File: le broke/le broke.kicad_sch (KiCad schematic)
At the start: 38 parts, among them SW1 SW_Push, U1 ProMicro

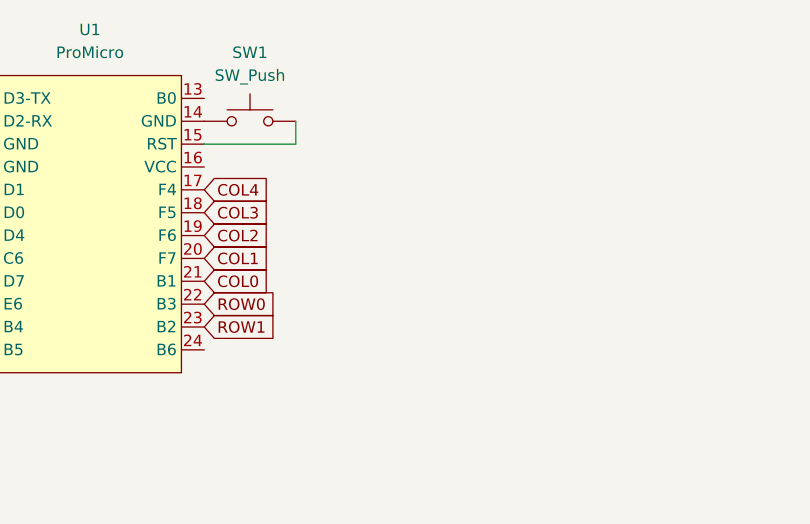
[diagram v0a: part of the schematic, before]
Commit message: new pcb etc
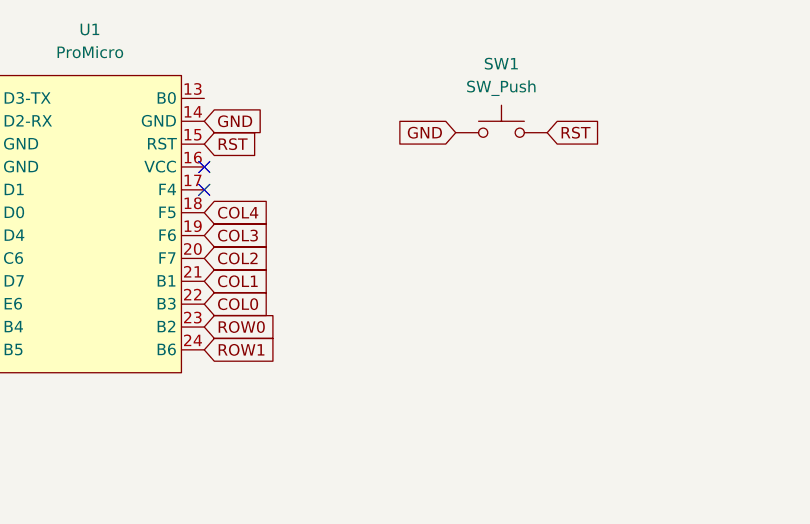
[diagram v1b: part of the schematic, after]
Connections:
- net COL0: now also U1.22 (B3); no longer U1.21 (B1)
- net COL1: now also U1.21 (B1); no longer U1.20 (F7)
- net COL2: now also U1.20 (F7); no longer U1.19 (F6)
- net COL3: now also U1.19 (F6); no longer U1.18 (F5)
- net COL4: now also U1.18 (F5); no longer U1.17 (F4)
- net ROW0: now also U1.23 (B2); no longer U1.22 (B3)
- net ROW1: now also U1.24 (B6); no longer U1.23 (B2)
- net GND: now reaches SW1.1, U1.14 (GND)
- net RST: now reaches SW1.2, U1.15 (RST)
- no-connect marks 0 -> 2
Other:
- moved on the sheet: SW1
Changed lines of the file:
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@@
 		(color 0 0 0 0)
 	)
+	(no_connect
+		(at 101.6 49.53)
+	)
+	(no_connect
+		(at 101.6 52.07)
+	)
 	(wire
 		(pts
@@
 	(wire
 		(pts
-			(xy 111.76 44.45) (xy 111.76 46.99)
-		)
-		(stroke
-			(width 0)
-			(type default)
-		)
-	)
-	(wire
-		(pts
 			(xy 139.7 116.84) (xy 139.7 142.24)
 		)
@@
 	(wire
 		(pts
-			(xy 111.76 46.99) (xy 101.6 46.99)
-		)
-		(stroke
-			(width 0)
-			(type default)
-		)
-	)
-	(wire
-		(pts
 			(xy 139.7 113.03) (xy 127 113.03)
 		)
@@
 	(global_label "ROW1"
 		(shape input)
+		(at 101.6 69.85 0)
+		(effects
+			(font
+				(size 1.27 1.27)
+			)
+			(justify left)
+		)
+		(property "Intersheetrefs" "${INTERSHEET_REFS}"
+			(at 101.6 69.85 0)
+			(effects
+				(font
+					(size 1.27 1.27)
+				)
+				(hide yes)
+			)
+		)
+	)
+	(global_label "ROW0"
+		(shape input)
 		(at 101.6 67.31 0)
 		(fields_autoplaced yes)
@@
 		)
 	)
+	(global_label "GND"
+		(shape input)
+		(at 101.6 44.45 0)
+		(effects
+			(font
+				(size 1.27 1.27)
+			)
+			(justify left)
+		)
+		(property "Intersheetrefs" "${INTERSHEET_REFS}"
+			(at 101.6 44.45 0)
+			(effects
+				(font
+					(size 1.27 1.27)
+				)
+				(hide yes)
+			)
+		)
+	)
 	(global_label "COL0"
 		(shape input)
@@
 		)
 	)
-	(global_label "ROW0"
+	(global_label "COL0"
 		(shape input)
 		(at 101.6 64.77 0)
@@
 		)
 	)
-	(global_label "COL2"
+	(global_label "COL3"
 		(shape input)
 		(at 101.6 57.15 0)
@@
 	(global_label "COL4"
 		(shape input)
-		(at 101.6 52.07 0)
+		(at 152.4 113.03 90)
 		(fields_autoplaced yes)
 		(effects
@@
 		)
 		(property "Intersheetrefs" "${INTERSHEET_REFS}"
-			(at 109.4233 52.07 0)
+			(at 152.4 105.2067 90)
 			(effects
 				(font
@@
 		)
 	)
-	(global_label "COL4"
+	(global_label "RST"
 		(shape input)
-		(at 152.4 113.03 90)
-		(fields_autoplaced yes)
+		(at 101.6 46.99 0)
 		(effects
 			(font
@@
 		)
 		(property "Intersheetrefs" "${INTERSHEET_REFS}"
-			(at 152.4 105.2067 90)
+			(at 101.6 46.99 0)
 			(effects
 				(font
 					(size 1.27 1.27)
 				)
-				(justify left)
 				(hide yes)
 			)
 		)
 	)
-	(global_label "COL0"
+	(global_label "COL1"
 		(shape input)
 		(at 101.6 62.23 0)
@@
 		)
 	)
-	(global_label "COL3"
+	(global_label "COL4"
 		(shape input)
 		(at 101.6 54.61 0)
@@
 		)
 	)
-	(global_label "COL1"
+	(global_label "COL2"
 		(shape input)
 		(at 101.6 59.69 0)
@@
 		)
 	)
+	(global_label "RST"
+		(shape input)
+		(at 139.7 45.72 0)
+		(effects
+			(font
+				(size 1.27 1.27)
+			)
+			(justify left)
+		)
+		(property "Intersheetrefs" "${INTERSHEET_REFS}"
+			(at 139.7 45.72 0)
+			(effects
+				(font
+					(size 1.27 1.27)
+				)
+				(hide yes)
+			)
+		)
+	)
+	(global_label "GND"
+		(shape input)
+		(at 129.54 45.72 180)
+		(effects
+			(font
+				(size 1.27 1.27)
+			)
+			(justify right)
+		)
+		(property "Intersheetrefs" "${INTERSHEET_REFS}"
+			(at 129.54 45.72 0)
+			(effects
+				(font
+					(size 1.27 1.27)
+				)
+				(hide yes)
+			)
+		)
+	)
 	(symbol
 		(lib_id "marbastlib-mx:MX_SW_solder")
@@
 	(symbol
 		(lib_id "Switch:SW_Push")
-		(at 106.68 44.45 0)
+		(at 134.62 45.72 0)
 		(unit 1)
 		(exclude_from_sim no)
@@
 		(fields_autoplaced yes)
 		(property "Reference" "SW1"
-			(at 106.68 36.83 0)
+			(at 134.62 38.1 0)
 			(effects
 				(font
@@
 		)
 		(property "Value" "SW_Push"
-			(at 106.68 39.37 0)
+			(at 134.62 40.64 0)
 			(effects
 				(font
@@
 		)
 		(property "Footprint" "Button_Switch_THT:SW_PUSH_6mm"
-			(at 106.68 39.37 0)
+			(at 134.62 40.64 0)
 			(effects
 				(font
@@
 		)
 		(property "Datasheet" "~"
-			(at 106.68 39.37 0)
+			(at 134.62 40.64 0)
 			(effects
 				(font
@@
 		)
 		(property "Description" "Push button switch, generic, two pins"
-			(at 106.68 44.45 0)
+			(at 134.62 45.72 0)
 			(effects
 				(font
